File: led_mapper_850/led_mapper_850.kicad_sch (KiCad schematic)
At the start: 555 parts, among them J1 Conn_02x12_Top_Bottom

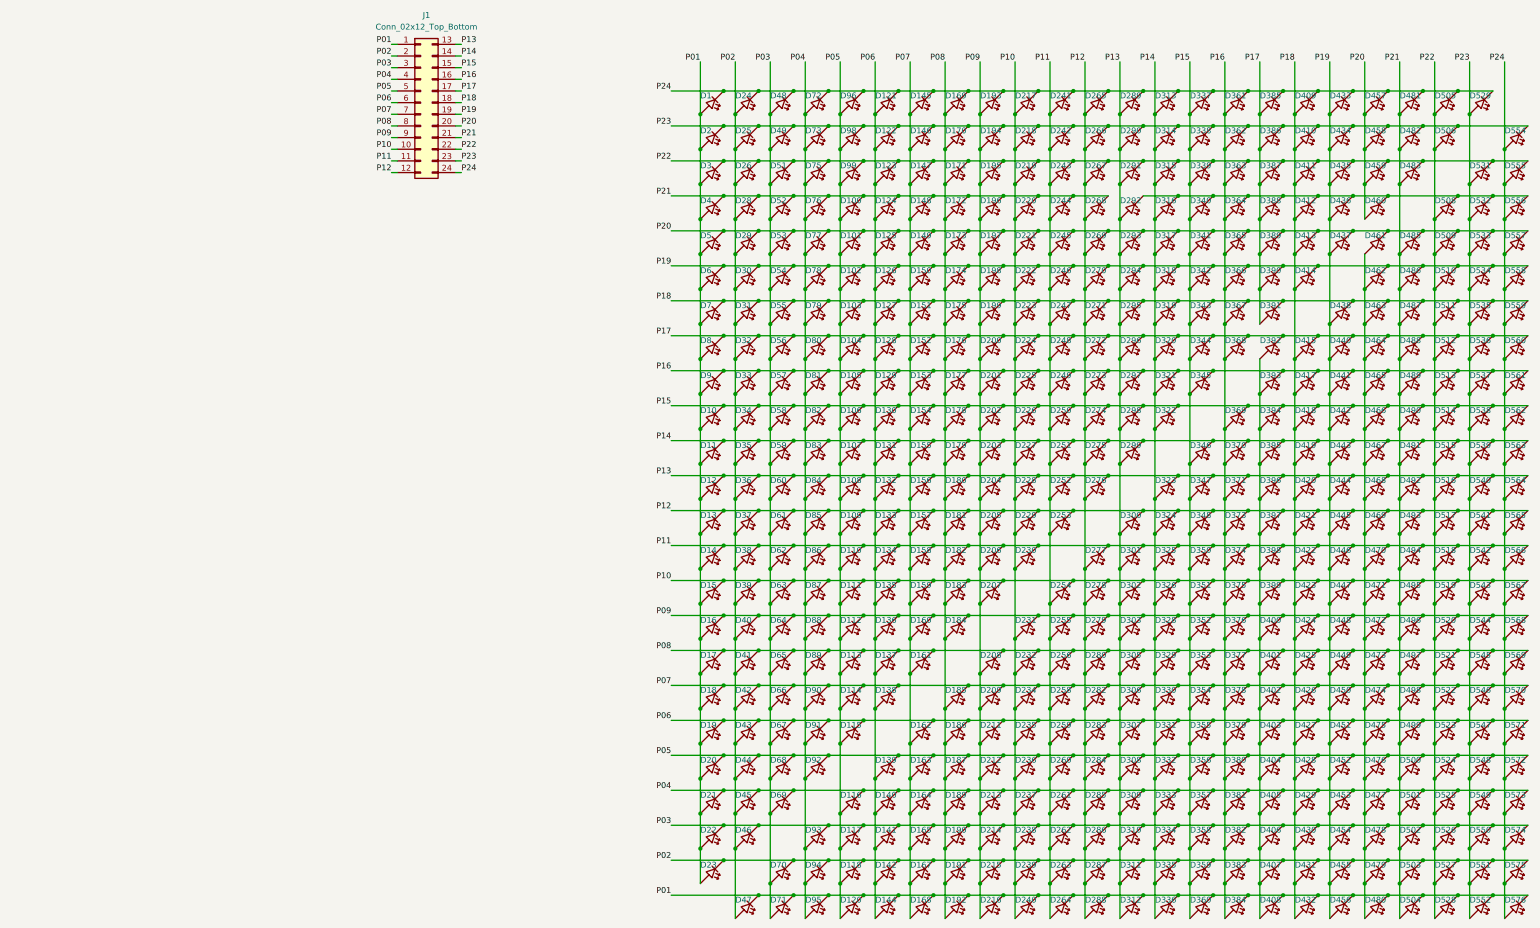
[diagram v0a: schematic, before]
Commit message: associate footprints
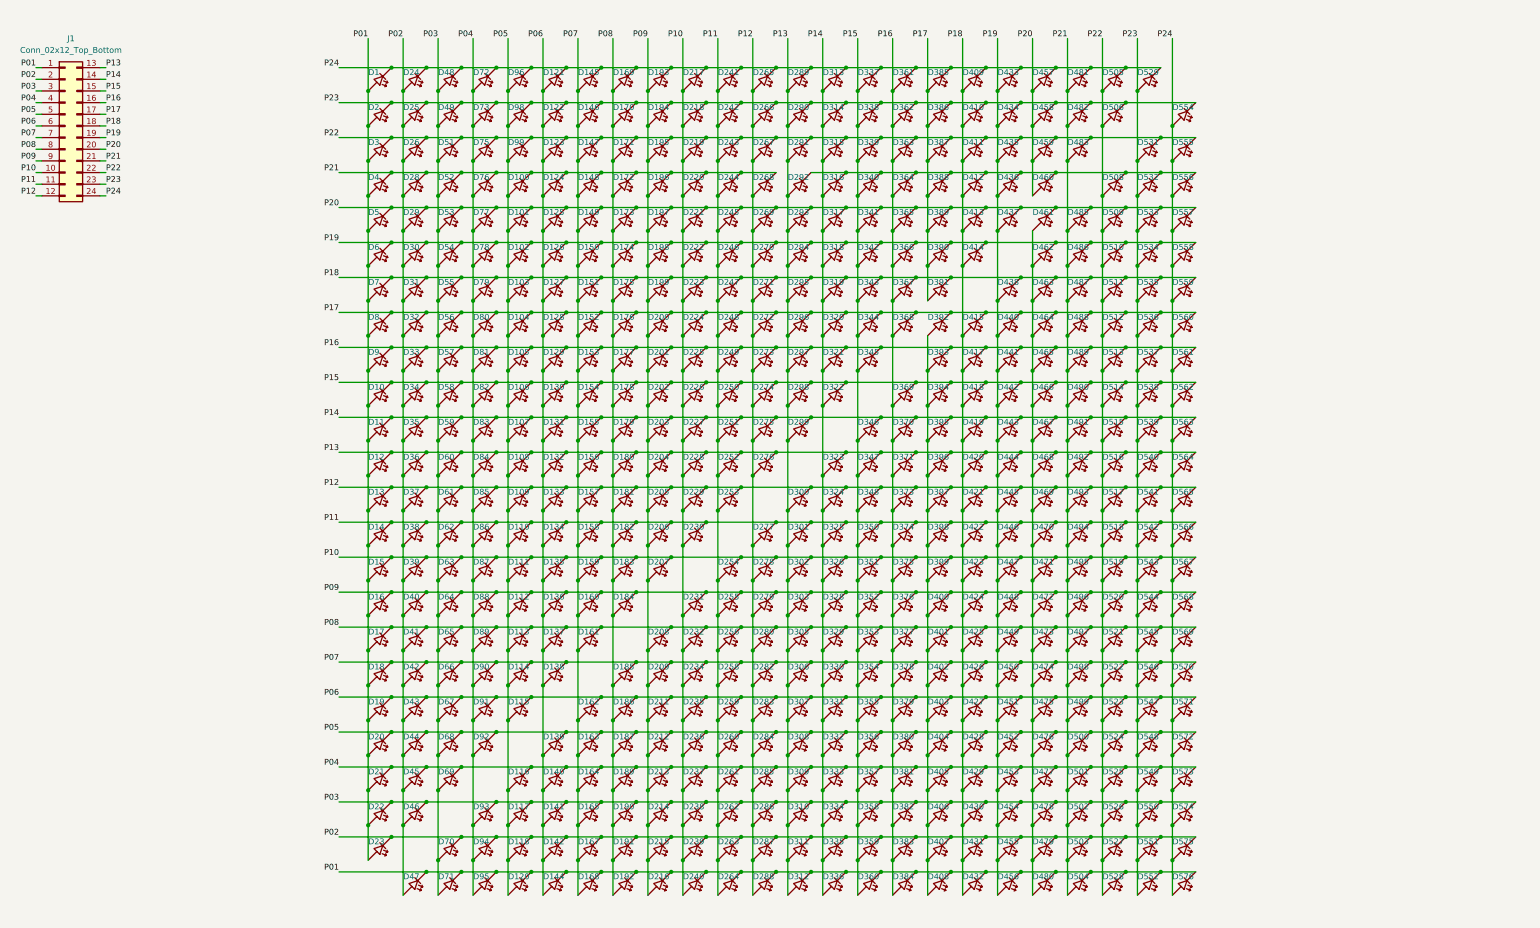
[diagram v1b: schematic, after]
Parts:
- D1, D10, D100, D101, D102, D103, D104, D105, D106, D107, D108, D109, D11, D110, D111, D112, D113, D114, D115, D116, D117, D118, D12, D120, D121, D122, D123, D124, D125, D126, D127, D128, D129, D13, D130, D131, D132, D133, D134, D135, D136, D137, D138, D139, D14, D140, D141, D142, D144, D145, D146, D147, D148, D149, D15, D150, D151, D152, D153, D154, D155, D156, D157, D158, D159, D16, D160, D161, D162, D163, D164, D165, D167, D168, D169, D17, D170, D171, D172, D173, D174, D175, D176, D177, D178, D179, D18, D180, D181, D182, D183, D184, D185, D186, D187, D189, D19, D190, D191, D192, D193, D194, D195, D196, D197, D198, D199, D2, D20, D200, D201, D202, D203, D204, D205, D206, D207, D208, D209, D21, D211, D212, D213, D214, D215, D216, D217, D218, D219, D22, D220, D221, D222, D223, D224, D225, D226, D227, D228, D229, D23, D230, D231, D232, D234, D235, D236, D237, D238, D239, D24, D240, D241, D242, D243, D244, D245, D246, D247, D248, D249, D25, D250, D251, D252, D253, D254, D255, D256, D258, D259, D26, D260, D261, D262, D263, D264, D265, D266, D267, D268, D269, D270, D271, D272, D273, D274, D275, D276, D277, D278, D279, D28, D280, D282, D283, D284, D285, D286, D287, D288, D289, D29, D290, D291, D292, D293, D294, D295, D296, D297, D298, D299, D3, D30, D300, D301, D302, D303, D305, D306, D307, D308, D309, D31, D310, D311, D312, D313, D314, D315, D316, D317, D318, D319, D32, D320, D321, D322, D323, D324, D325, D326, D328, D329, D33, D330, D331, D332, D333, D334, D335, D336, D337, D338, D339, D34, D340, D341, D342, D343, D344, D345, D346, D347, D348, D35, D350, D351, D352, D353, D354, D355, D356, D357, D358, D359, D36, D360, D361, D362, D363, D364, D365, D366, D367, D368, D369, D37, D370, D371, D373, D374, D375, D376, D377, D378, D379, D38, D380, D381, D382, D383, D384, D385, D386, D387, D388, D389, D39, D390, D391, D392, D393, D394, D395, D396, D397, D398, D399, D4, D40, D400, D401, D402, D403, D404, D405, D406, D407, D408, D409, D41, D410, D411, D412, D413, D414, D415, D417, D418, D419, D42, D420, D421, D422, D423, D424, D425, D426, D427, D428, D429, D43, D430, D431, D432, D433, D434, D435, D436, D437, D438, D44, D440, D441, D442, D443, D444, D445, D446, D447, D448, D449, D45, D450, D451, D452, D453, D454, D455, D456, D457, D458, D459, D46, D460, D461, D462, D463, D464, D465, D466, D467, D468, D469, D47, D470, D471, D472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: footprint (none) -> LED_SMD:LED_0201_0603Metric
- J1: footprint (none) -> ccatlib:PinSocket_2x12_P2.54mm_Vertical_SMD_custom
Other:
- moved on the sheet: D1, D10, D100, D101, D102, D103, D104, D105, D106, D107, D108, D109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
